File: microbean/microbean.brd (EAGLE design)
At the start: 30.5 x 27.6 mm, 17 parts, among them IC2 MAX485ST3485, IC3 PIC16F1827SO

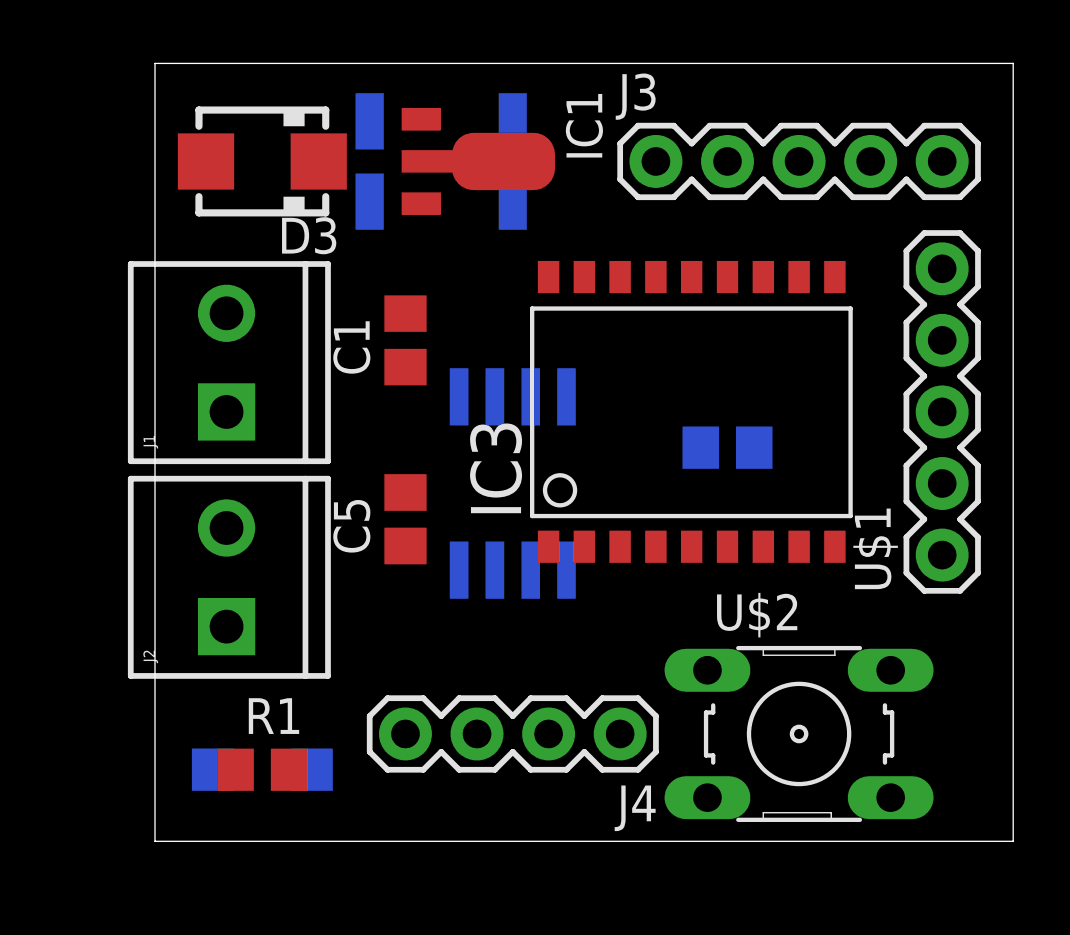
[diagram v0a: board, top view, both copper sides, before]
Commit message: - WIP microbean for professional printing
git-svn-id: svn://mule/net/hardware/trunk@556 1a6b750e-079f-425f-90e7-3a118970be6b
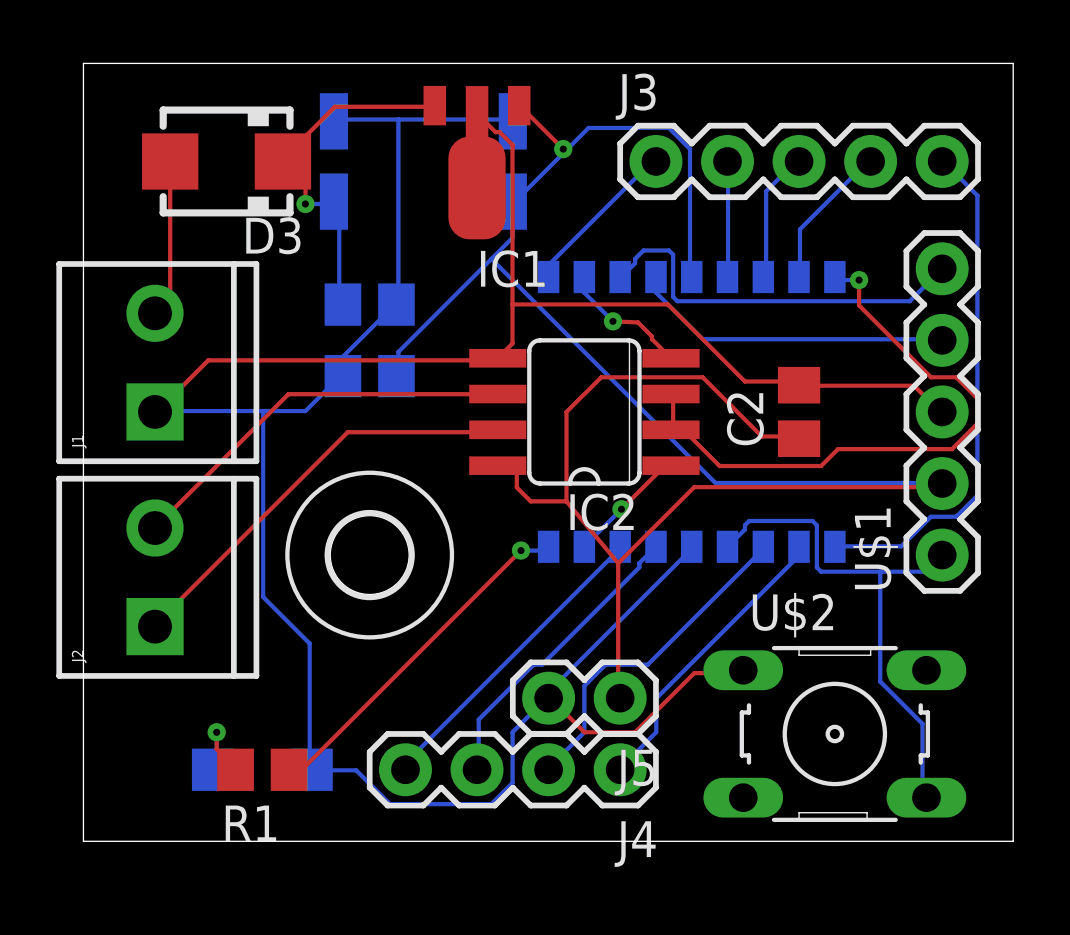
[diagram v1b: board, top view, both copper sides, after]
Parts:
- added J5: (no value), custom:1X02
- added U$4: (no value), holes:2,8
- moved C5 5.24 mm to (11.4, 27.9), flipped to the bottom, turned to 0 degrees
- moved IC2 3.59 mm to (19.1, 26.7), flipped to the top, turned to 90 degrees
- moved C2 2.84 mm to (26.7, 26.7), flipped to the top, turned to 90 degrees
- moved J1 2.54 mm to (3.81, 26.7)
- moved J2 2.54 mm to (3.81, 19.1)
- moved C1 1.80 mm to (11.4, 30.5), flipped to the bottom, turned to 180 degrees
- moved D3 1.27 mm to (6.35, 35.6)
- moved C3 1.27 mm to (10.2, 35.6)
- moved J4 1.27 mm to (20.3, 14.0)
- moved U$2 1.27 mm to (27.9, 15.2)
- turned C4 to 270 degrees
- turned IC1 to 180 degrees
- flipped IC3 to the bottom
- turned R1 to 180 degrees
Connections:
- net GND: now also J5.2
- net N$10: now also R1.2; no longer R1.1
- net N$13: now also J5.1
- net N$14: now also IC3.7; no longer IC3.1
- net N$15: now also IC3.6; no longer IC3.2
- net N$17: now also IC3.2; no longer IC3.6
- net N$18: now also IC3.1; no longer IC3.7
- net N$19: now also IC3.17; no longer IC3.9
- net N$20: now also IC3.16; no longer IC3.10
- net N$21: now also IC3.10; no longer IC3.15
- net N$4: now also IC3.15; no longer IC3.16
- net N$9: now also IC3.9, R1.1; no longer IC3.17, R1.2
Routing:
- net GND: track 0.00 -> 103.6 mm
- net N$13: track 0.00 -> 79.3 mm, vias 0 -> 1
- net N$23: track 0.00 -> 21.7 mm, vias 0 -> 1
- net N$6: track 0.00 -> 18.7 mm
- net N$18: track 0.00 -> 18.2 mm
- net N$3: track 0.00 -> 15.2 mm
- net N$5: track 0.00 -> 14.1 mm
- net N$8: track 0.00 -> 14.0 mm
- net N$2: track 0.00 -> 12.9 mm, vias 0 -> 1
- net N$9: track 0.00 -> 12.5 mm, vias 0 -> 1
- net N$16: track 0.00 -> 11.9 mm
- net N$7: track 0.00 -> 11.4 mm
- net N$14: track 0.00 -> 11.1 mm
- net N$15: track 0.00 -> 10.7 mm
- net N$17: track 0.00 -> 10.5 mm
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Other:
- board size 30.5 x 27.6 mm -> 33 x 27.6 mm
